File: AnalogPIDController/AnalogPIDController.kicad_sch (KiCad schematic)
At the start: 7 parts, among them U1 TL082

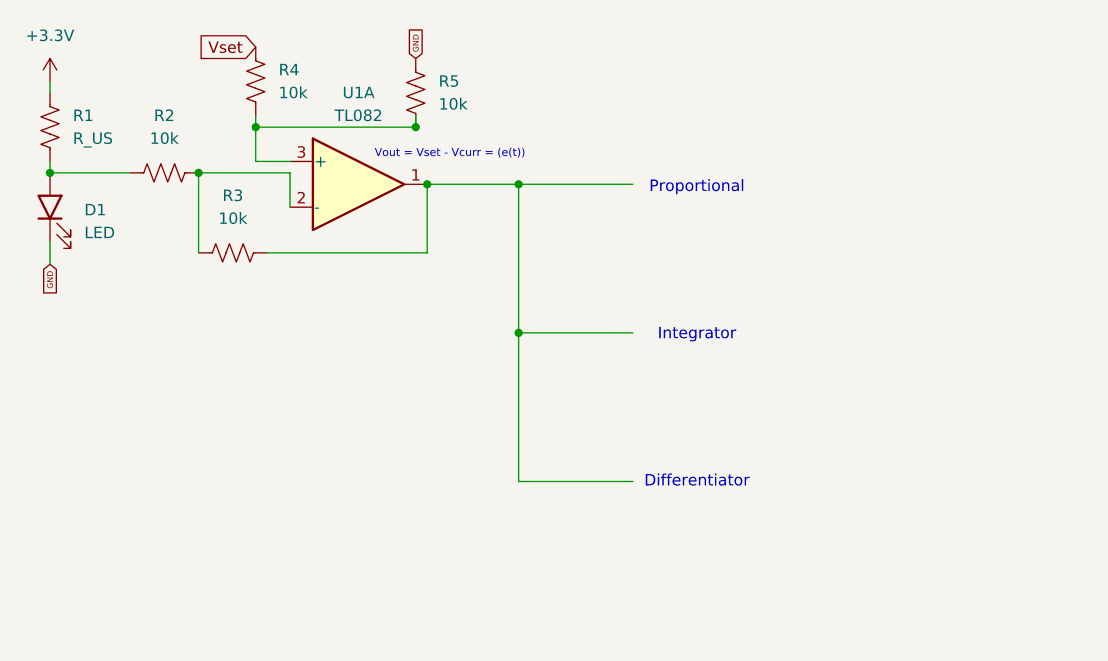
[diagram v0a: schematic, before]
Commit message: Finished Some of PID schematic
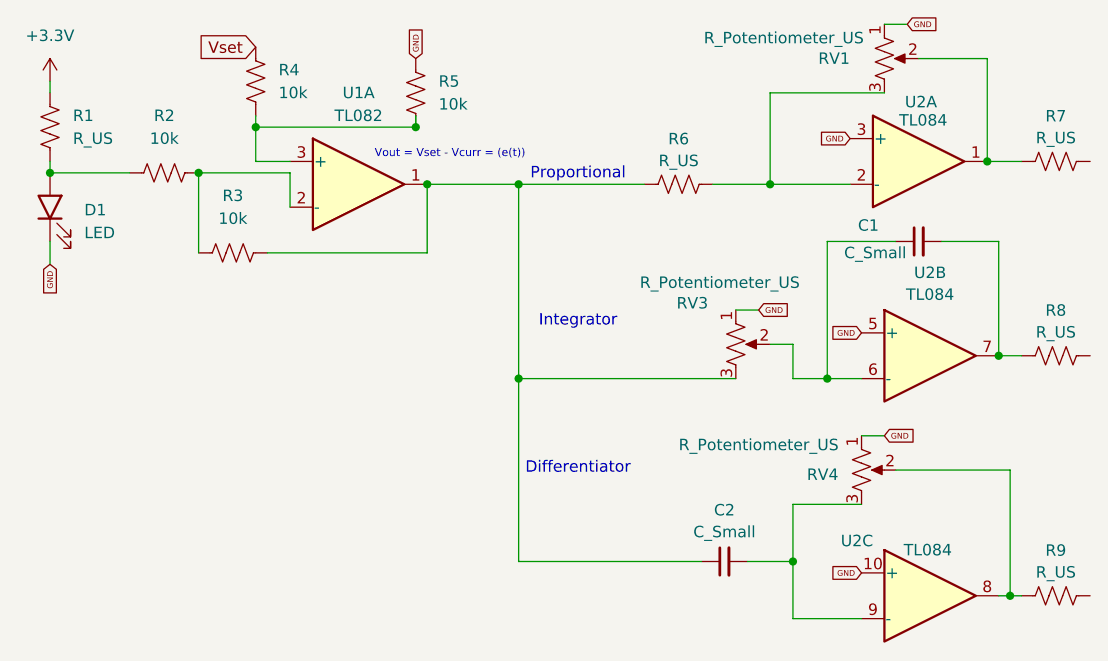
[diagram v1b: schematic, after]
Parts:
- added C1, C2: C_Small, symbol Device:C_Small
- added R6, R7, R8, R9: R_US, symbol Device:R_US
- added RV1, RV3, RV4: R_Potentiometer_US, symbol Device:R_Potentiometer_US
- added U2: TL084, symbol Amplifier_Operational:TL084
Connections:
- net GND: now also RV1.1, RV3.1, RV4.1, U2.10 (+), U2.3 (+), U2.5 (+)
- net at R3.1, U1.1: now also C2.1, R6.1, RV3.3
- new net: C1.1, RV3.2, U2.6 (-)
- new net: C1.2, R8.1, U2.7
- new net: R9.1, RV4.2, U2.8
- new net: C2.2, RV4.3, U2.9 (-)
- new net: R7.1, RV1.2, U2.1
- new net: R6.2, RV1.3, U2.2 (-)
